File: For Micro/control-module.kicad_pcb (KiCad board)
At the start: 2 copper layers, 25 parts, among them J1 For Light Sensor, J2 For Light Sensor, J3 From Solar Panel, J4 For Flow Module b, J5 For Flow Module a, Q1 NMOS, Q2 NMOS, U1 STR05, U2 ARDUINO_MICRO_SHIELD

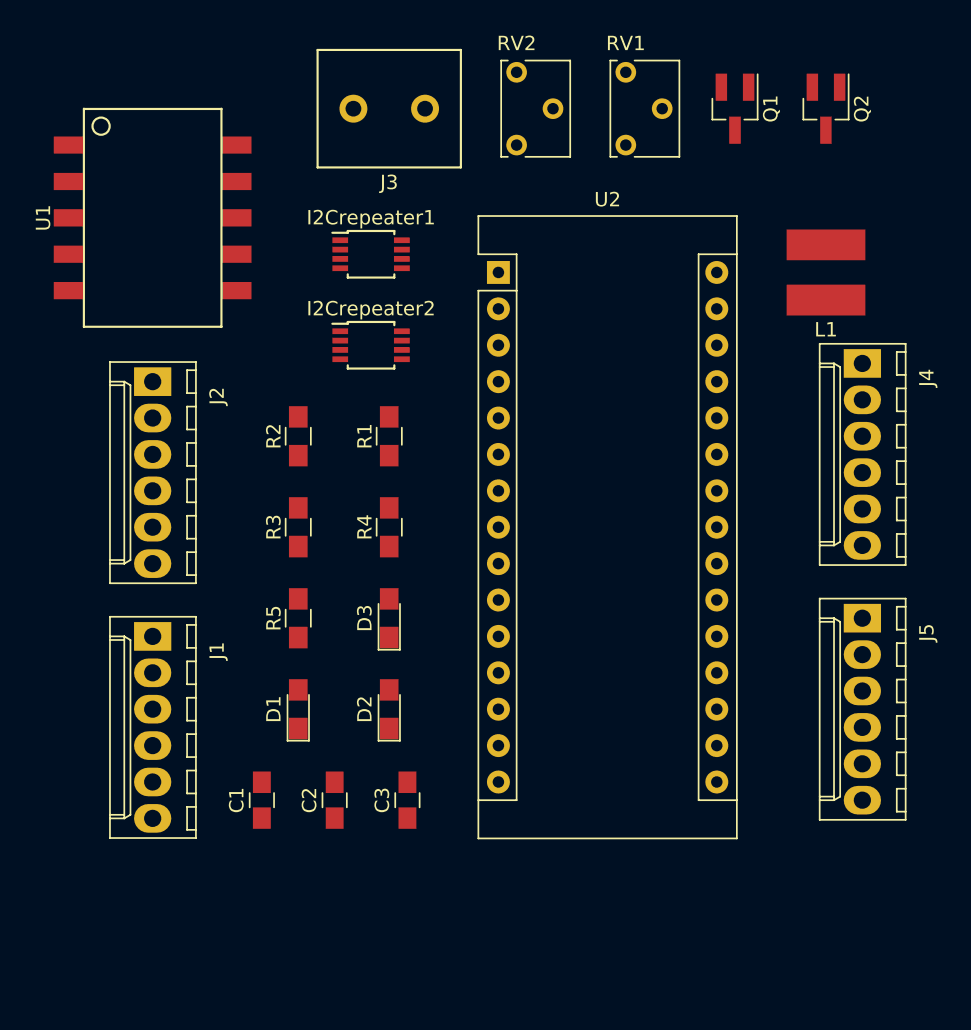
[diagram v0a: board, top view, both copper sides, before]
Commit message: PCB for Control
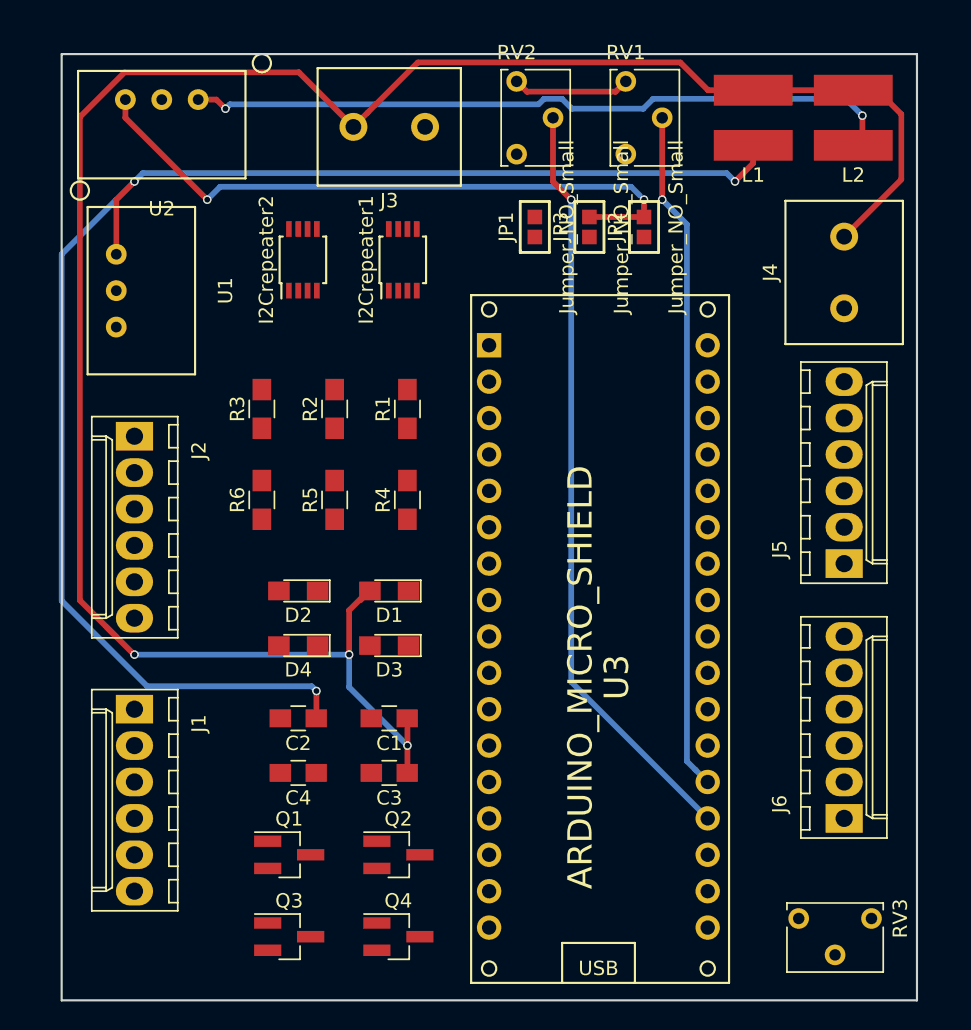
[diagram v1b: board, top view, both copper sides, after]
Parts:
- added C4: 10uF, Capacitors_SMD:C_0805_HandSoldering, F.Cu at (104.1, 137.8)
- added D4: LED, LEDs:LED_0805_HandSoldering, F.Cu at (104.1, 128.9)
- added J6: For Flow Module a, valveteam-footprints:Molex_KK-6410-06_06x2.54mm_Straight, F.Cu at (142.2, 141.0)
- added JP1: Jumper_NO_Small, valveteam-footprints:SMD-solder-bridge, F.Cu at (120.7, 99.7)
- added JP2: Jumper_NO_Small, valveteam-footprints:SMD-solder-bridge, F.Cu at (128.3, 99.7)
- added JP3: Jumper_NO_Small, valveteam-footprints:SMD-solder-bridge, F.Cu at (124.5, 99.7)
- added L2: 6.8uH, valveteam-footprints:WURTH_INDUCTOR, F.Cu at (142.9, 92.1)
- added Q3: NMOS, TO_SOT_Packages_SMD:SOT-23_Handsoldering, F.Cu at (103.5, 149.2)
- added Q4: NMOS, TO_SOT_Packages_SMD:SOT-23_Handsoldering, F.Cu at (111.1, 149.2)
- added R6: 470, Resistors_SMD:R_0805_HandSoldering, F.Cu at (101.6, 118.7)
- added RV3: Trimmer Upper, Potentiometers:Potentiometer_Trimmer_Vishay_T73XX_Vertical, F.Cu at (144.1, 148.0)
- added U3: ARDUINO_MICRO_SHIELD, valveteam-footprints:ARDUINO_MICRO_SHIELD, F.Cu at (116.2, 104.5)
- C1, C2, C3: value 4.7uF -> 10uF
- J1: value For Light Sensor -> For Expansion
- J4: value For Flow Module b -> To Flow Module (F); footprint valveteam-footprints:Molex_KK-6410-06_06x2.54mm_Straight -> valveteam-footprints:TE_TERM
- J5: value For Flow Module a -> For Flow Module b
- L1: value 3.3uH -> 6.8uH
- R4, R5: value 150 -> 470
- U1: value STR05 -> TR_SERIES; footprint valveteam-footprints:STR05 -> valveteam-footprints:TR_Series
- U2: value ARDUINO_MICRO_SHIELD -> TR_SERIES; footprint valveteam-footprints:Arduino_Nano -> valveteam-footprints:TR_Series
- moved Q1 60.7 mm to (103.5, 143.5), turned to 0 degrees
- moved Q2 60.0 mm to (111.1, 143.5), turned to 0 degrees
- moved U2 26.4 mm to (94.6, 90.8)
- moved L1 11.9 mm to (135.9, 92.1)
- moved C1 10.6 mm to (110.5, 134.0), turned to 180 degrees
- moved D1 10.4 mm to (110.5, 125.1), turned to 180 degrees
- moved D2 10.4 mm to (104.1, 125.1), turned to 180 degrees
- moved R3 8.64 mm to (101.6, 112.4)
- moved R5 8.64 mm to (106.7, 118.7)
- moved I2Crepeater2 7.62 mm to (104.5, 102.0), turned to 90 degrees
- moved J4 6.48 mm to (142.2, 102.9)
- moved C2 6.25 mm to (104.1, 134.0), turned to 180 degrees
- moved U1 5.68 mm to (91.4, 104.1), turned to 90 degrees
- moved J1 5.24 mm to (92.7, 133.3)
- moved J2 4.02 mm to (92.7, 114.3)
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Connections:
- C2 pad 1: 12V -> Net-(C2-Pad1)
- C3 pad 1: Net-(C3-Pad1) -> 12V
- D1 pad 1: GND -> Net-(D1-Pad1)
- D1 pad 2: Net-(D1-Pad2) -> 12V
- D3 pad 1: GND -> Net-(D3-Pad1)
- D3 pad 2: Net-(D3-Pad2) -> VCC+5V
- J1 pad 1: VCC+3V -> VCC+EXP
- J2 pad 1: VCC+3V -> VCC+LS
- J4 pad 1: VCC+5V -> 12V
- J4 pad 2: INPUT2 -> GND
- J5 pad 2: Net-(J5-Pad2) -> INPUT2
- J5 pad 5: Net-(J5-Pad5) -> INPUT5
- L1 pad 2: Net-(L1-Pad2) -> Net-(C2-Pad1)
- Q1 pad 1: INT -> EN1
- Q1 pad 2: INT/M -> EN1/M
- Q2 pad 1: DVI -> EN2
- Q2 pad 2: DVI/M -> EN2/M
- R3 pad 1: 12V -> Net-(D1-Pad1)
- R3 pad 2: Net-(D1-Pad2) -> GND
- R5 pad 1: VCC+5V -> Net-(D3-Pad1)
- R5 pad 2: Net-(D3-Pad2) -> GND
- U1 pad VI: Net-(L1-Pad2) -> Net-(C2-Pad1)
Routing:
- net 12V: track 0.00 -> 146.6 mm, vias 0 -> 3
- net Net-(C2-Pad1): track 0.00 -> 104.7 mm, vias 0 -> 3
- net A0: track 0.00 -> 53.4 mm, vias 0 -> 1
- net Net-(C4-Pad1): track 0.00 -> 50.3 mm, vias 0 -> 2
- net A1: track 0.00 -> 47.7 mm, vias 0 -> 1
- net VCC+3V: track 0.00 -> 45.2 mm, vias 0 -> 2
- net 5V: track 0.00 -> 8.22 mm
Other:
- board outline added: 59.7 x 66 mm
- net class Default: trace_width 0.25 -> 0.4
